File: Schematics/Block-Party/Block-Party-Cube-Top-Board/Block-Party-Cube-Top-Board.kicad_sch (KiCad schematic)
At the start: 5 parts

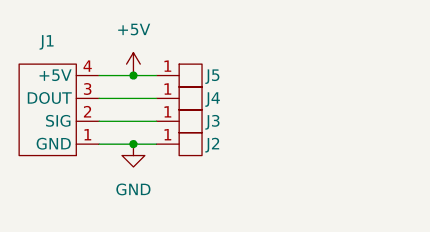
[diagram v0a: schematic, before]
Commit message: Revision 1.01 of the PCBs
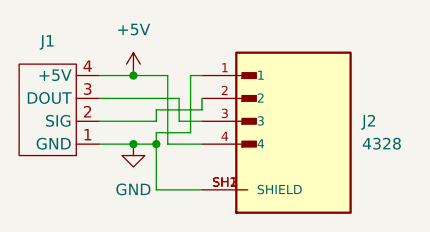
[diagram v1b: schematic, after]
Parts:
- removed J2, J3, J4, J5: ~, Connector_PinHeader_2.54mm:PinHeader_1x01_P2.54mm_Vertical, symbol Quinn_lib:HDR-M-2.54_1x1
- added J2: 4328, adafruit-jst-4328:ADAFRUIT_4328, symbol 4328:4328
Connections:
- net +5V: now also J2.4
- net GND: now also J2.1, J2.SH1 (SHIELD), J2.SH2 (SHIELD)
- net at J1.2 (SIG): now also J2.2
- net at J1.3 (DOUT): now also J2.3
